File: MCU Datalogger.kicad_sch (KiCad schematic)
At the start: 25 parts, among them U1 24LC1025, U2 DS1337S_, U3 24LC1025, U4 ATMEGA328P-AU, Y1 32.768 KHz, Y2 16 MHz

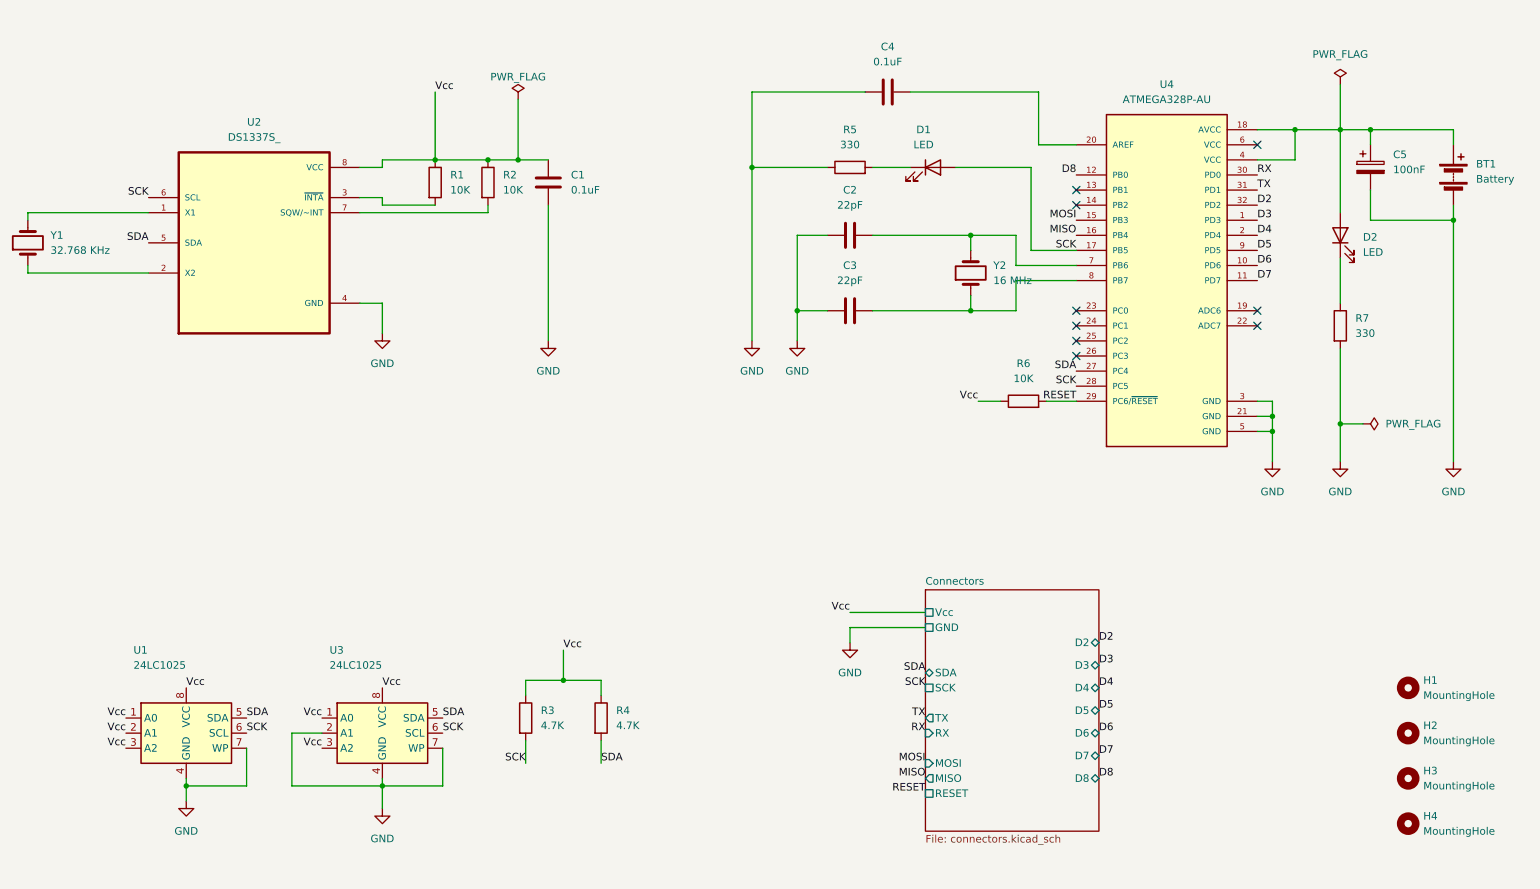
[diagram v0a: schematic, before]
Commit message: Added comments.
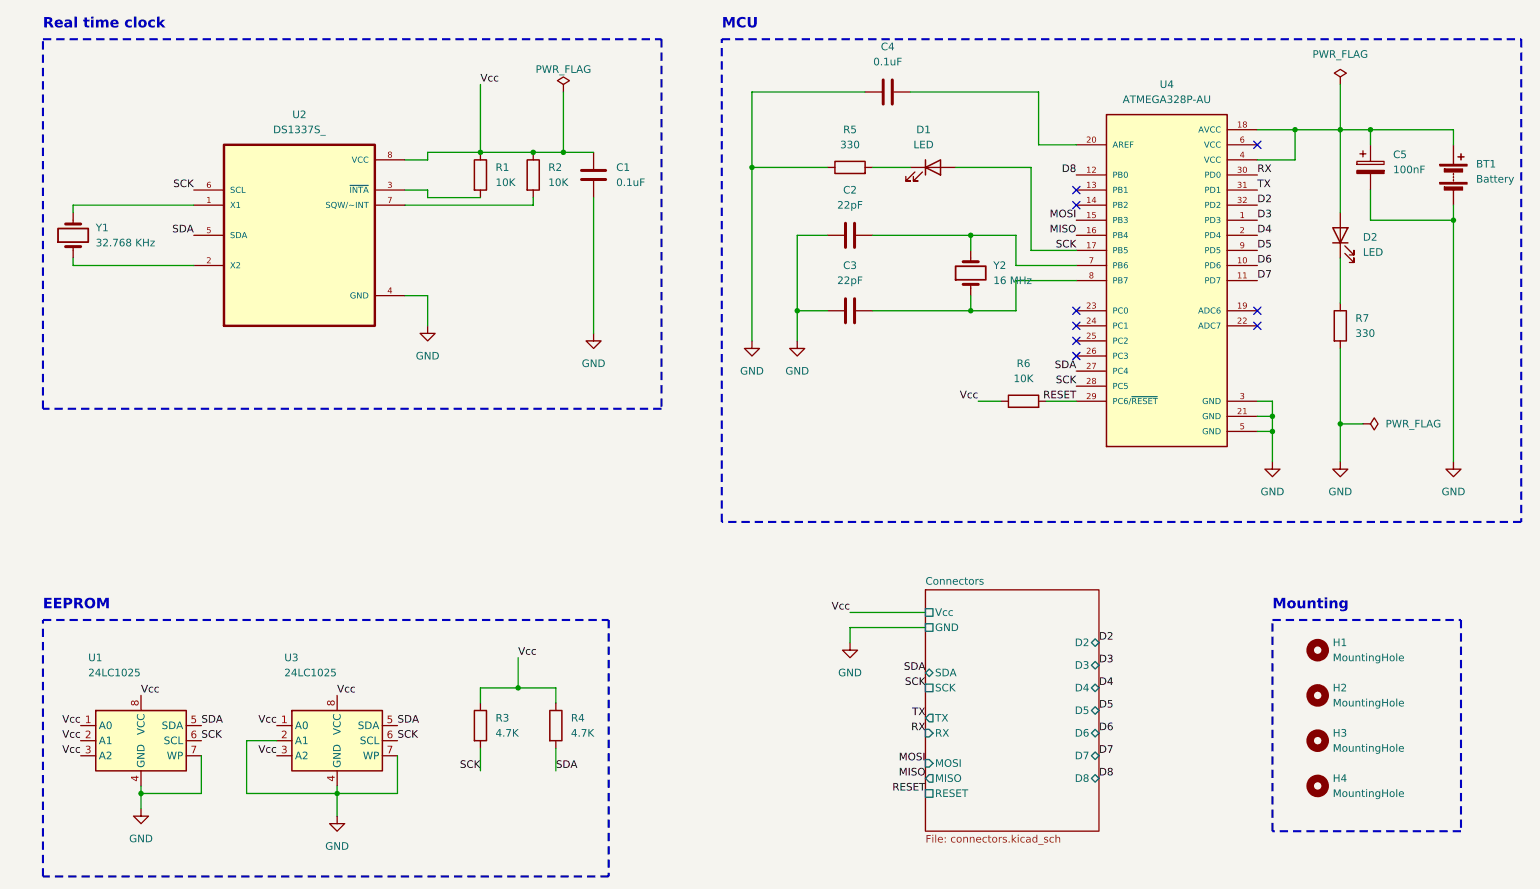
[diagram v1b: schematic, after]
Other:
- note added: "EEPROM"
- note added: "MCU"
- note added: "Mounting"
- note added: "Real time clock"
- moved on the sheet: C1, H1, H2, H3, H4, R1, R2, R3, R4, U1, U2, U3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
